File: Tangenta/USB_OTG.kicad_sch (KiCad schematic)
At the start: 21 parts, among them J11 TYPEC-304-ACP16, U10 TUSB321RWBR, U11 AOZ1353DI-01, U12 PUSB2X4Y-N, U9 PUSB2X4Y-N

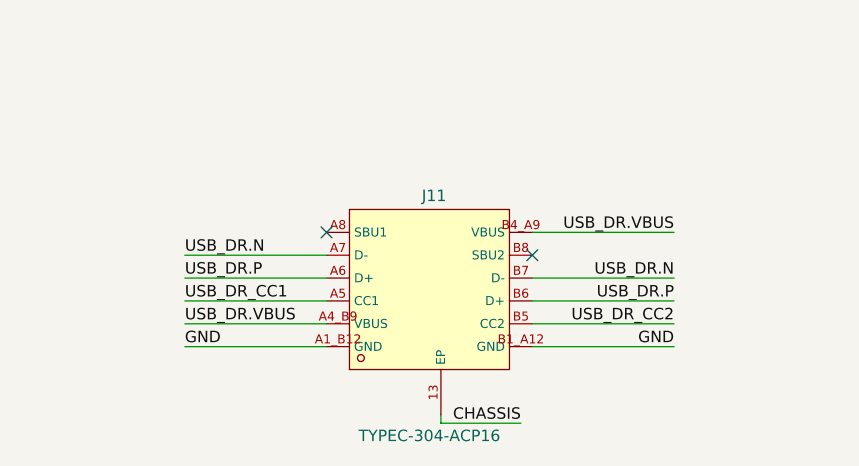
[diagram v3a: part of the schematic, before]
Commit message: ...
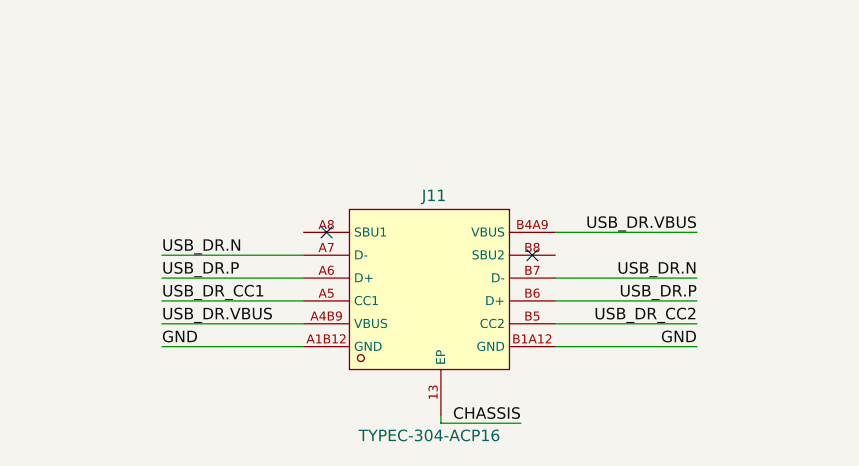
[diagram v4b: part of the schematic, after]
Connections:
- net GNDREF: now also J11.A1B12 (GND), J11.B1A12 (GND); no longer J11.A1_B12 (GND), J11.B1_A12 (GND)
- net USB_DR.VBUS: now also J11.A4B9 (VBUS), J11.B4A9 (VBUS); no longer J11.A4_B9 (VBUS), J11.B4_A9 (VBUS)
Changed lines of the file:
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@@
     (stroke (width 0) (type default))
   )
-  (wire (pts (xy 102.108 142.494) (xy 86.36 142.494))
+  (wire (pts (xy 99.568 142.494) (xy 83.82 142.494))
     (stroke (width 0) (type default))
   )
@@
     (stroke (width 0) (type default))
   )
-  (wire (pts (xy 124.968 150.114) (xy 140.716 150.114))
+  (wire (pts (xy 127.508 150.114) (xy 143.256 150.114))
     (stroke (width 0) (type default))
   )
@@
     (stroke (width 0) (type default))
   )
-  (wire (pts (xy 102.108 145.034) (xy 86.36 145.034))
+  (wire (pts (xy 99.568 145.034) (xy 83.82 145.034))
     (stroke (width 0) (type default))
   )
@@
     (stroke (width 0) (type default))
   )
-  (wire (pts (xy 124.968 152.654) (xy 140.716 152.654))
+  (wire (pts (xy 127.508 152.654) (xy 143.256 152.654))
     (stroke (width 0) (type default))
   )
@@
     (stroke (width 0) (type default))
   )
-  (wire (pts (xy 102.108 152.654) (xy 86.36 152.654))
+  (wire (pts (xy 99.568 152.654) (xy 83.82 152.654))
     (stroke (width 0) (type default))
   )
@@
     (stroke (width 0) (type default))
   )
-  (wire (pts (xy 124.968 139.954) (xy 140.716 139.954))
+  (wire (pts (xy 127.508 139.954) (xy 143.256 139.954))
     (stroke (width 0) (type default))
   )
@@
     (stroke (width 0) (type default))
   )
-  (wire (pts (xy 124.968 145.034) (xy 140.716 145.034))
+  (wire (pts (xy 127.508 145.034) (xy 143.256 145.034))
     (stroke (width 0) (type default))
   )
@@
     (stroke (width 0) (type default))
   )
-  (wire (pts (xy 86.36 150.114) (xy 102.108 150.114))
+  (wire (pts (xy 83.82 150.114) (xy 99.568 150.114))
     (stroke (width 0) (type default))
   )
@@
     (stroke (width 0) (type default))
   )
-  (wire (pts (xy 102.108 147.574) (xy 86.36 147.574))
+  (wire (pts (xy 99.568 147.574) (xy 83.82 147.574))
     (stroke (width 0) (type default))
   )
@@
     (stroke (width 0) (type default))
   )
-  (wire (pts (xy 124.968 147.574) (xy 140.716 147.574))
+  (wire (pts (xy 127.508 147.574) (xy 143.256 147.574))
     (stroke (width 0) (type default))
   )
@@
     (effects (font (size 1.27 1.27)) (justify right bottom))
   )
-  (label "USB_DR.P" (at 86.36 145.034 0) (fields_autoplaced)
+  (label "USB_DR.P" (at 83.82 145.034 0) (fields_autoplaced)
     (effects (font (size 1.27 1.27)) (justify left bottom))
   )
@@
     (effects (font (size 1.27 1.27)) (justify left bottom))
   )
-  (label "USB_DR.N" (at 86.36 142.494 0) (fields_autoplaced)
+  (label "USB_DR.N" (at 83.82 142.494 0) (fields_autoplaced)
     (effects (font (size 1.27 1.27)) (justify left bottom))
   )
@@
     (effects (font (size 1.27 1.27)) (justify left bottom))
   )
-  (label "USB_DR.N" (at 140.716 145.034 180) (fields_autoplaced)
-    (effects (font (size 1.27 1.27)) (justify right bottom))
-  )
-  (label "GND" (at 86.36 152.654 0) (fields_autoplaced)
+  (label "USB_DR.N" (at 143.256 145.034 180) (fields_autoplaced)
+    (effects (font (size 1.27 1.27)) (justify right bottom))
+  )
+  (label "GND" (at 83.82 152.654 0) (fields_autoplaced)
     (effects (font (size 1.27 1.27)) (justify left bottom))
   )
@@
     (effects (font (size 1.27 1.27)) (justify left bottom))
   )
-  (label "USB_DR_CC2" (at 140.716 150.114 180) (fields_autoplaced)
+  (label "USB_DR_CC2" (at 143.256 150.114 180) (fields_autoplaced)
     (effects (font (size 1.27 1.27)) (justify right bottom))
   )
@@
     (effects (font (size 1.27 1.27)) (justify right bottom))
   )
-  (label "USB_DR.VBUS" (at 86.36 150.114 0) (fields_autoplaced)
+  (label "USB_DR.VBUS" (at 83.82 150.114 0) (fields_autoplaced)
     (effects (font (size 1.27 1.27)) (justify left bottom))
   )
@@
     (effects (font (size 1.27 1.27)) (justify right bottom))
   )
-  (label "USB_DR.VBUS" (at 140.716 139.954 180) (fields_autoplaced)
+  (label "USB_DR.VBUS" (at 143.256 139.954 180) (fields_autoplaced)
     (effects (font (size 1.27 1.27)) (justify right bottom))
   )
@@
     (effects (font (size 1.27 1.27)) (justify right bottom))
   )
-  (label "USB_DR_CC1" (at 86.36 147.574 0) (fields_autoplaced)
+  (label "USB_DR_CC1" (at 83.82 147.574 0) (fields_autoplaced)
     (effects (font (size 1.27 1.27)) (justify left bottom))
   )
@@
     (effects (font (size 1.27 1.27)) (justify right bottom))
   )
-  (label "GND" (at 140.716 152.654 180) (fields_autoplaced)
-    (effects (font (size 1.27 1.27)) (justify right bottom))
-  )
-  (label "USB_DR.P" (at 140.716 147.574 180) (fields_autoplaced)
+  (label "GND" (at 143.256 152.654 180) (fields_autoplaced)
+    (effects (font (size 1.27 1.27)) (justify right bottom))
+  )
+  (label "USB_DR.P" (at 143.256 147.574 180) (fields_autoplaced)
     (effects (font (size 1.27 1.27)) (justify right bottom))
   )
@@
     )
     (pin "13")
-    (pin "A1_B12")
-    (pin "A4_B9")
+    (pin "A1B12")
+    (pin "A4B9")
     (pin "A5")
     (pin "A6")
     (pin "A7")
     (pin "A8")
-    (pin "B1_A12")
-    (pin "B4_A9")
+    (pin "B1A12")
+    (pin "B4A9")
     (pin "B5")
     (pin "B6")
